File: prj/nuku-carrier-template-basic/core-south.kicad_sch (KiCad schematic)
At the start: 19 parts, among them J1 DF40HC(4.0)-90DS-0.4V, SW1 PROG

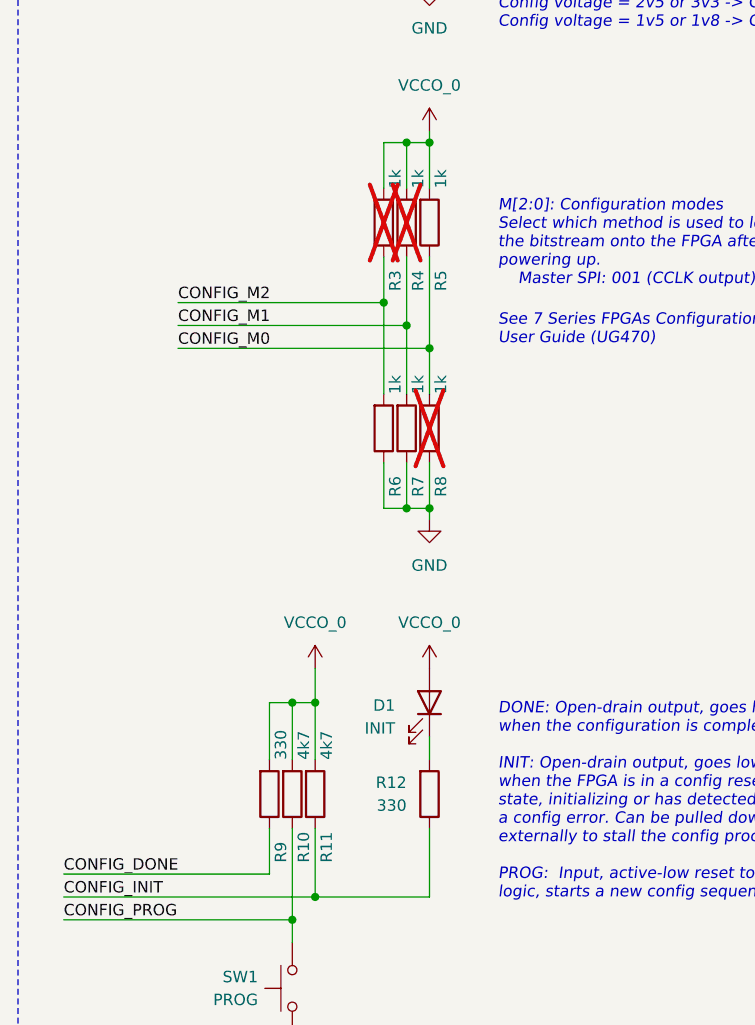
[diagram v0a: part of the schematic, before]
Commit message: Route template.basic
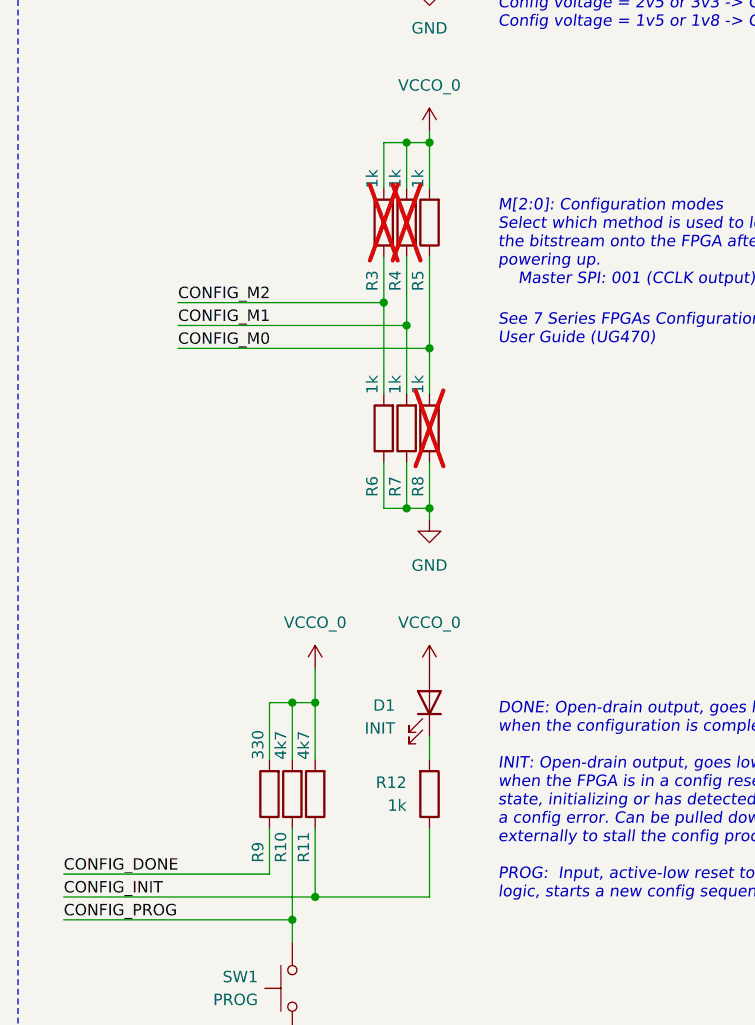
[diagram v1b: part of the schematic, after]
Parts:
- R12: value 330 -> 1k; LCSC C25104 -> C11702
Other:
- moved on the sheet: R10, R11, R3, R4, R5, R6, R7, R8, R9
